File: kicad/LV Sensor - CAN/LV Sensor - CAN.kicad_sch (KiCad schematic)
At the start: 4 parts, among them U1 ATA00F18S-L, U2 MCP251863T-H-SS, U3 DSC1001DL5-020.0000T

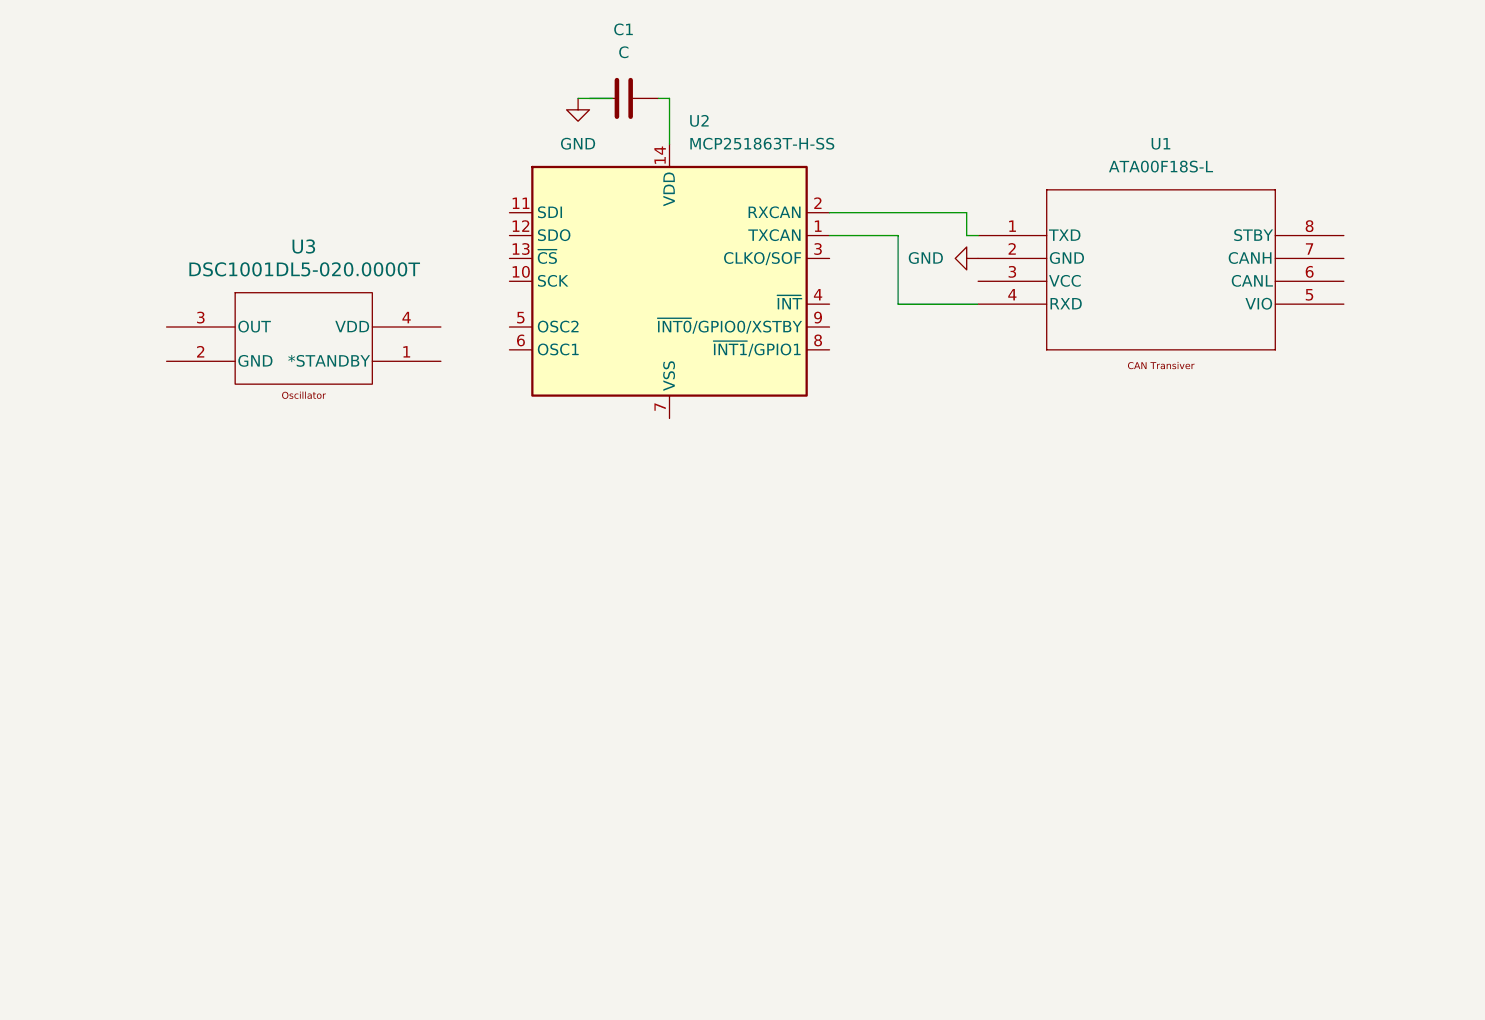
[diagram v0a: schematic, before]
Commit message: 09-05-2025 "Finished" LV-Sensor-Can Board
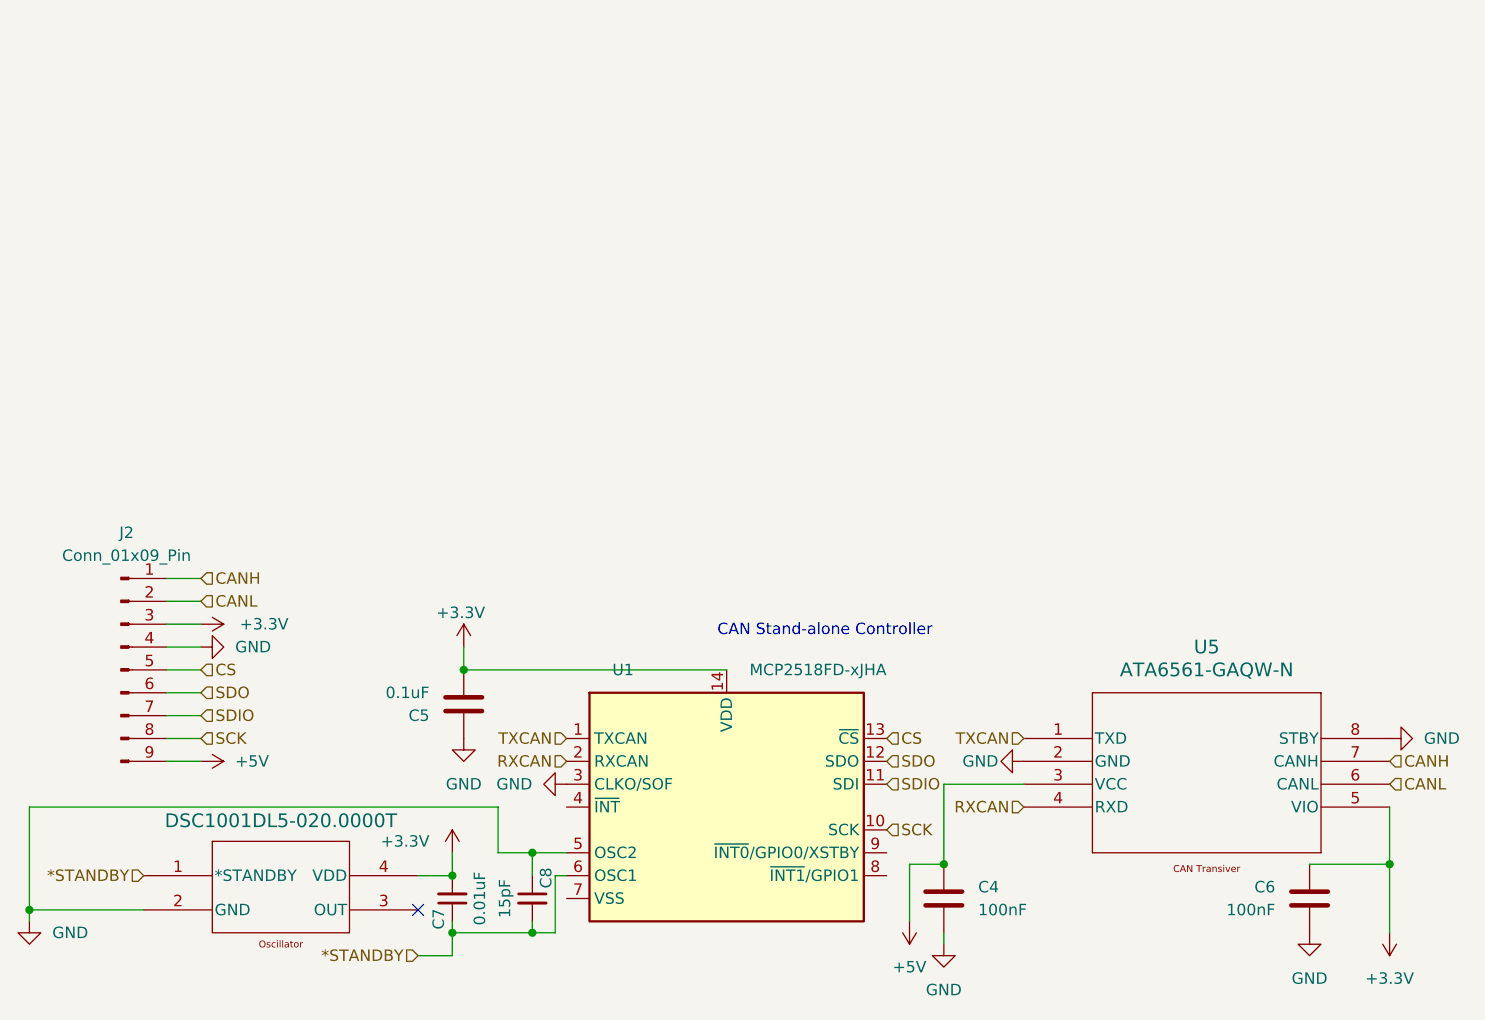
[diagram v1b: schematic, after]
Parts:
- removed C1: C, symbol Device:C
- removed U1: ATA00F18S-L, LV-Sensor-Footprints-Lib:SOIC8_4P9X3P9MC_MCH, symbol LV-Sensor-Lib:ATA6561-GAQW-N
- removed U2: MCP251863T-H-SS, LV-Sensor-Footprints-Lib:MCP2518FDT, symbol LV-Sensor-Lib:MCP2517FD-xJHA
- removed U3: DSC1001DL5-020.0000T, LV-Sensor-Footprints-Lib:CDFN4_2P5X2_MCH, symbol LV-Sensor-Lib:DSC1001DL5-020.0000T
- added C4, C6: 100nF, Capacitor_SMD:C_1206_3216Metric_Pad1.33x1.80mm_HandSolder, symbol Device:C
- added C5: 0.1uF, Capacitor_SMD:C_1206_3216Metric_Pad1.33x1.80mm_HandSolder, symbol Device:C
- added C7: 0.01uF, Capacitor_SMD:C_1206_3216Metric_Pad1.33x1.80mm_HandSolder, symbol Device:C_Small
- added C8: 15pF, Capacitor_SMD:C_1206_3216Metric_Pad1.33x1.80mm_HandSolder, symbol Device:C_Small
- added J2: Conn_01x09_Pin, Connector_PinHeader_2.54mm:PinHeader_1x09_P2.54mm_Vertical, symbol Connector:Conn_01x09_Pin
- added U1: MCP2518FD-xJHA, LV-Sensor-Footprints-Lib:MCP2518FDT, symbol LV-Sensor-Lib:MCP2517FD-xJHA
- added U2: DSC1001DL5-020.0000T, LV-Sensor-Footprints-Lib:CDFN4_2P5X2_MCH, symbol LV-Sensor-Lib:DSC1001DL5-020.0000T
- added U5: ATA6561-GAQW-N, LV-Sensor-Footprints-Lib:SOIC8_4P9X3P9MC_MCH, symbol LV-Sensor-Lib:ATA6561-GAQW-N
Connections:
- net GND: now also C4.2, C5.1, C6.2, C8.1, J2.4 (Pin_4), U1.3 (CLKO/SOF), U1.5 (OSC2), U2.2 (GND), U5.2 (GND), U5.8 (STBY)
- new net *STANDBY: C7.1, C8.2, U1.6 (OSC1), U2.1 (*STANDBY)
- new net +3.3V: C5.2, C6.1, C7.2, J2.3 (Pin_3), U1.14 (VDD), U2.4 (VDD), U5.5 (VIO)
- new net +5V: C4.1, J2.9 (Pin_9), U5.3 (VCC)
- new net CANH: J2.1 (Pin_1), U5.7 (CANH)
- new net CANL: J2.2 (Pin_2), U5.6 (CANL)
- new net CS: J2.5 (Pin_5), U1.13 (~{CS})
- new net RXCAN: U1.2 (RXCAN), U5.4 (RXD)
- new net SCK: J2.8 (Pin_8), U1.10 (SCK)
- new net SDIO: J2.7 (Pin_7), U1.11 (SDI)
- new net SDO: J2.6 (Pin_6), U1.12 (SDO)
- new net TXCAN: U1.1 (TXCAN), U5.1 (TXD)
- no-connect marks 0 -> 1
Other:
- note added: "CAN Stand-alone Controller"
